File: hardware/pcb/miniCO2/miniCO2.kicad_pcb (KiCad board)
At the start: 4 copper layers, 13.7 x 15.7 mm, 11 parts, among them J1 USB_A, SW1 SW_Push, U1 ATSAMD21E18A-M, U2 AP2112K-3.3, U3 SCD40-D-R2

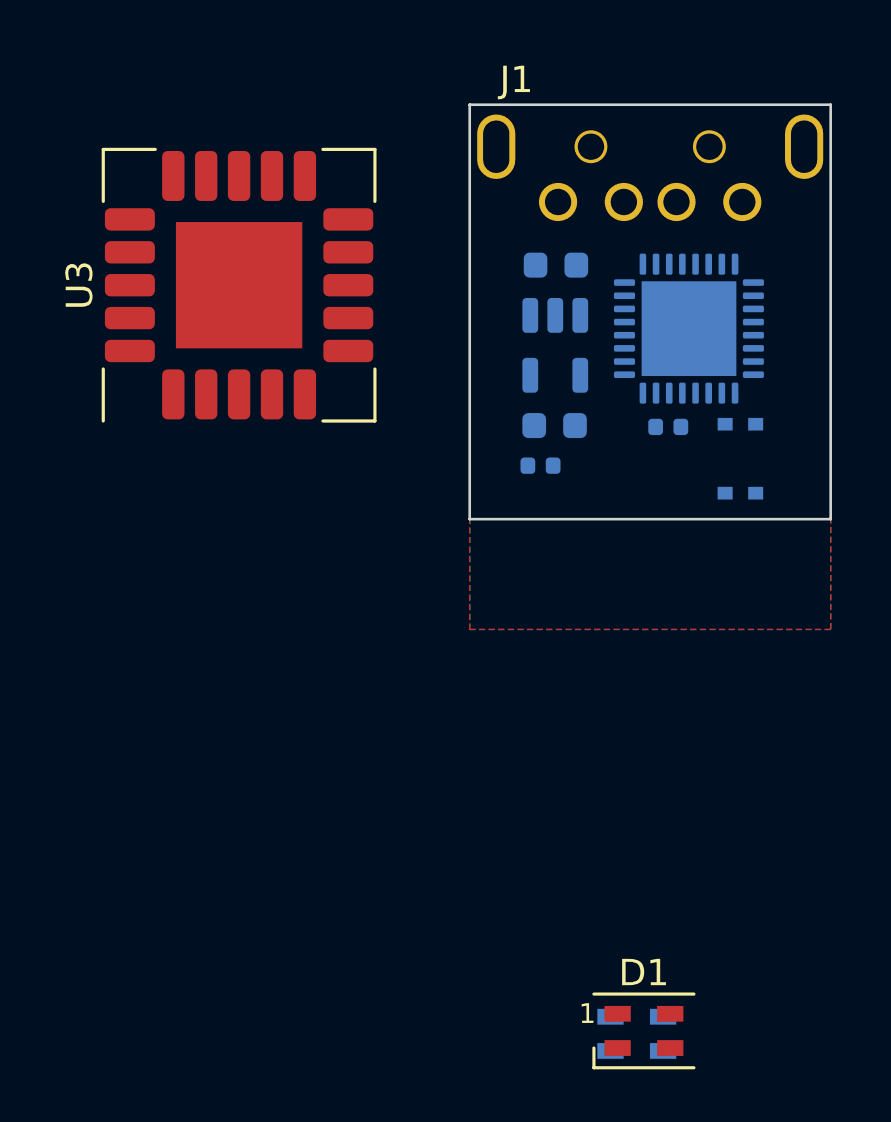
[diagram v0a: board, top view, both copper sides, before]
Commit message: Routing finished
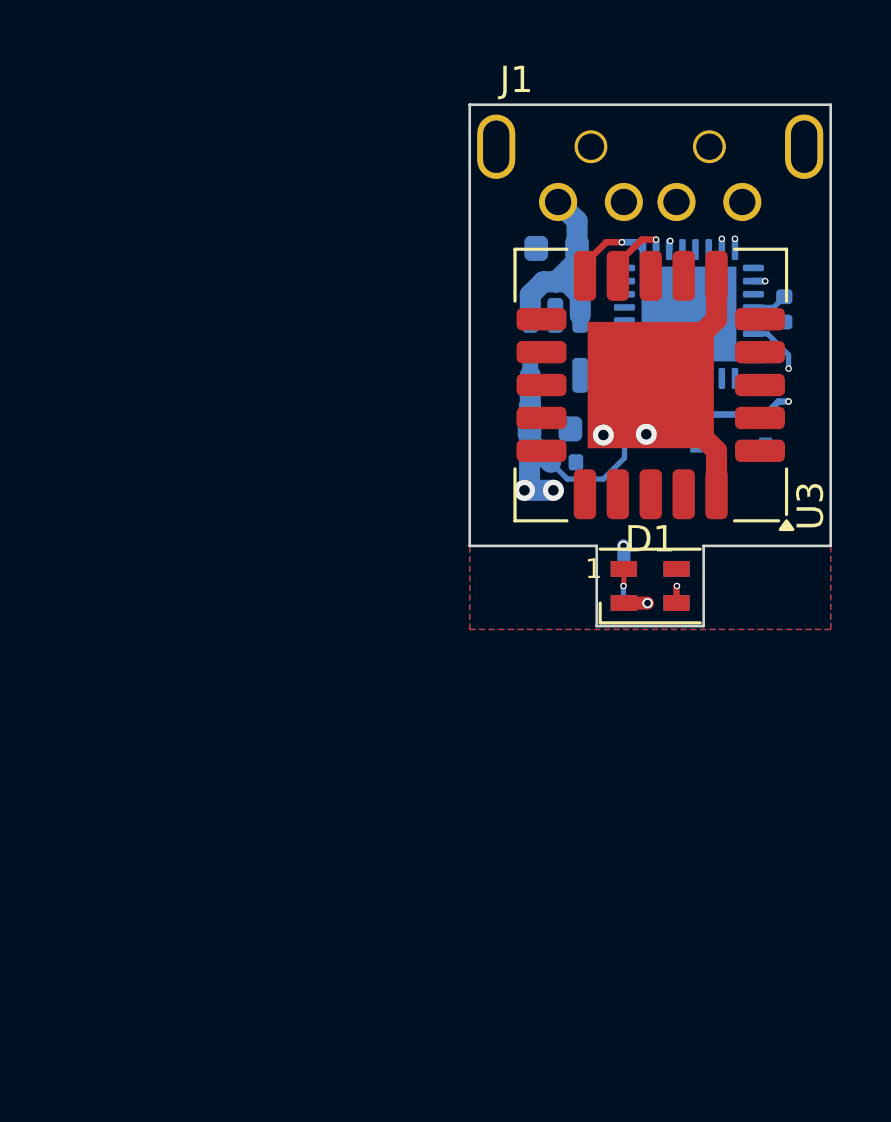
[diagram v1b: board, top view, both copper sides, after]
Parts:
- D1, D2: footprint LED_SMD:LED_SK6805_PLCC4_2.4x2.7mm_P1.3mm -> miniCO2:LED_SK6805_PLCC4_2.4x2.7mm_P1.3mm
- U1: footprint Package_DFN_QFN:QFN-32-1EP_5x5mm_P0.5mm_EP3.6x3.6mm -> miniCO2:QFN-32-1EP_5x5mm_P0.5mm_EP3.6x3.6mm
- U3: footprint Sensor:Sensirion_SCD4x-1EP_10.1x10.1mm_P1.25mm_EP4.8x4.8mm -> miniCO2:Sensirion_SCD4x-1EP_10.1x10.1mm_P1.25mm_EP4.8x4.8mm
- moved D2 17.0 mm to (141.5, 97.5)
- moved D1 16.9 mm to (141.5, 97.5)
- moved U3 16.1 mm to (141.5, 89.9), turned to 180 degrees
- moved C4 6.28 mm to (146.6, 87.0), turned to -90 degrees
- moved SW1 1.16 mm to (144.6, 91.6), turned to 0 degrees
- moved C3 0.88 mm to (138.2, 92.8)
- moved C1 0.64 mm to (137.9, 84.7), turned to 0 degrees
- moved U1 0.56 mm to (143.0, 87.2), turned to 90 degrees
- moved C2 0.22 mm to (137.7, 91.6)
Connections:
- U1 pad 19: unconnected-(U1-PA18-Pad19) -> DIN
- U1 pad 31: unconnected-(U1-PA30-Pad31) -> SWCLK
- U1 pad 32: unconnected-(U1-PA31-Pad32) -> SWDIO
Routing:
- net +3.3V: track 0.00 -> 17.4 mm, vias 0 -> 4
- net GND: track 0.00 -> 17.2 mm, vias 0 -> 3
- net DIN: track 0.00 -> 14.2 mm, vias 0 -> 2
- net Net-(U1-~{RESET}): track 0.00 -> 9.09 mm, vias 0 -> 2
- net VBUS: track 0.00 -> 7.53 mm
- net D-: track 0.00 -> 4.71 mm, vias 0 -> 1
- net D+: track 0.00 -> 3.33 mm, vias 0 -> 1
- net SDA: track 0.00 -> 3.12 mm, vias 0 -> 1
- net SCL: track 0.00 -> 2.67 mm, vias 0 -> 1
- net Net-(D1-DOUT): track 0.00 -> 1.31 mm, vias 0 -> 1
- net Net-(U1-VDDCORE): track 0.00 -> 1.20 mm
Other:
- board size 13.7 x 15.7 mm -> 13.7 x 19.8 mm
